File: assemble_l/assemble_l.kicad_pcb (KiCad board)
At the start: 2 copper layers, 134.9 x 119.3 mm, 61 parts, among them J1 Conn_01x02_Pin, SW1 SW_Push, SW10 SW_Push, SW11 SW_Push, SW12 SW_Push, SW13 SW_Push, SW14 SW_Push, SW15 SW_Push, SW16 SW_Push, SW17 SW_Push, SW18 SW_Push, SW19 SW_Push, SW2 SW_Push, SW20 SW_Push, SW21 SW_Push, SW22 SW_Push, SW23 SW_Push, SW24 SW_Push, SW25 SW_Push, SW26 SW_Push, SW27 SW_Push, SW28 SW_Push, SW3 SW_Push, SW4 SW_Push, SW5 SW_Push, SW6 SW_Push, SW7 SW_Push, SW8 SW_Push, SW9 SW_Push, U1 Micon_BLEMicroPro

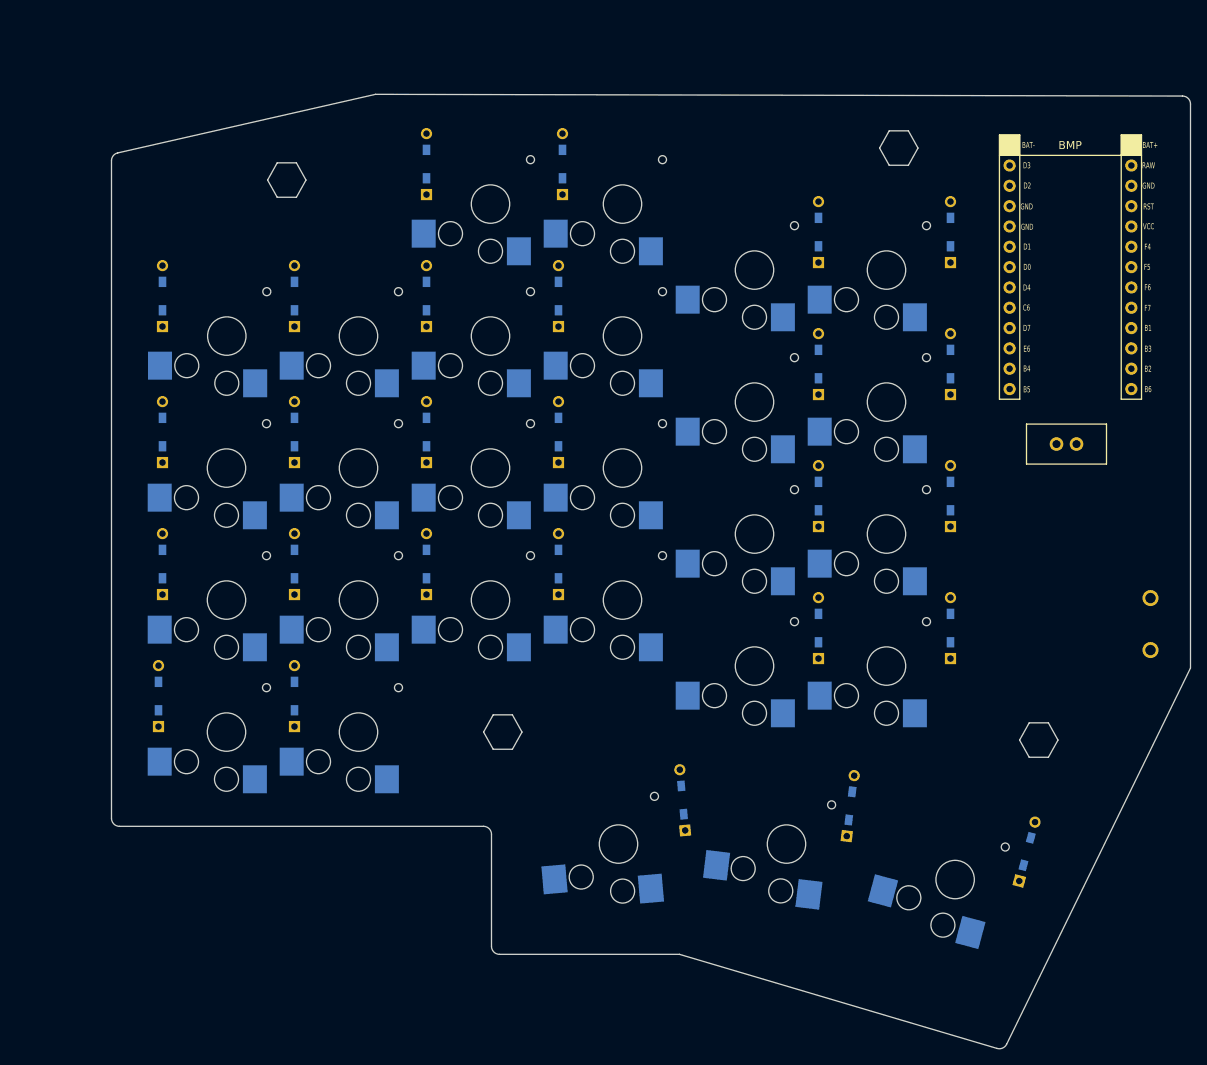
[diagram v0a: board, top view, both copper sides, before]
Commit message: feat: reallocate keys on left
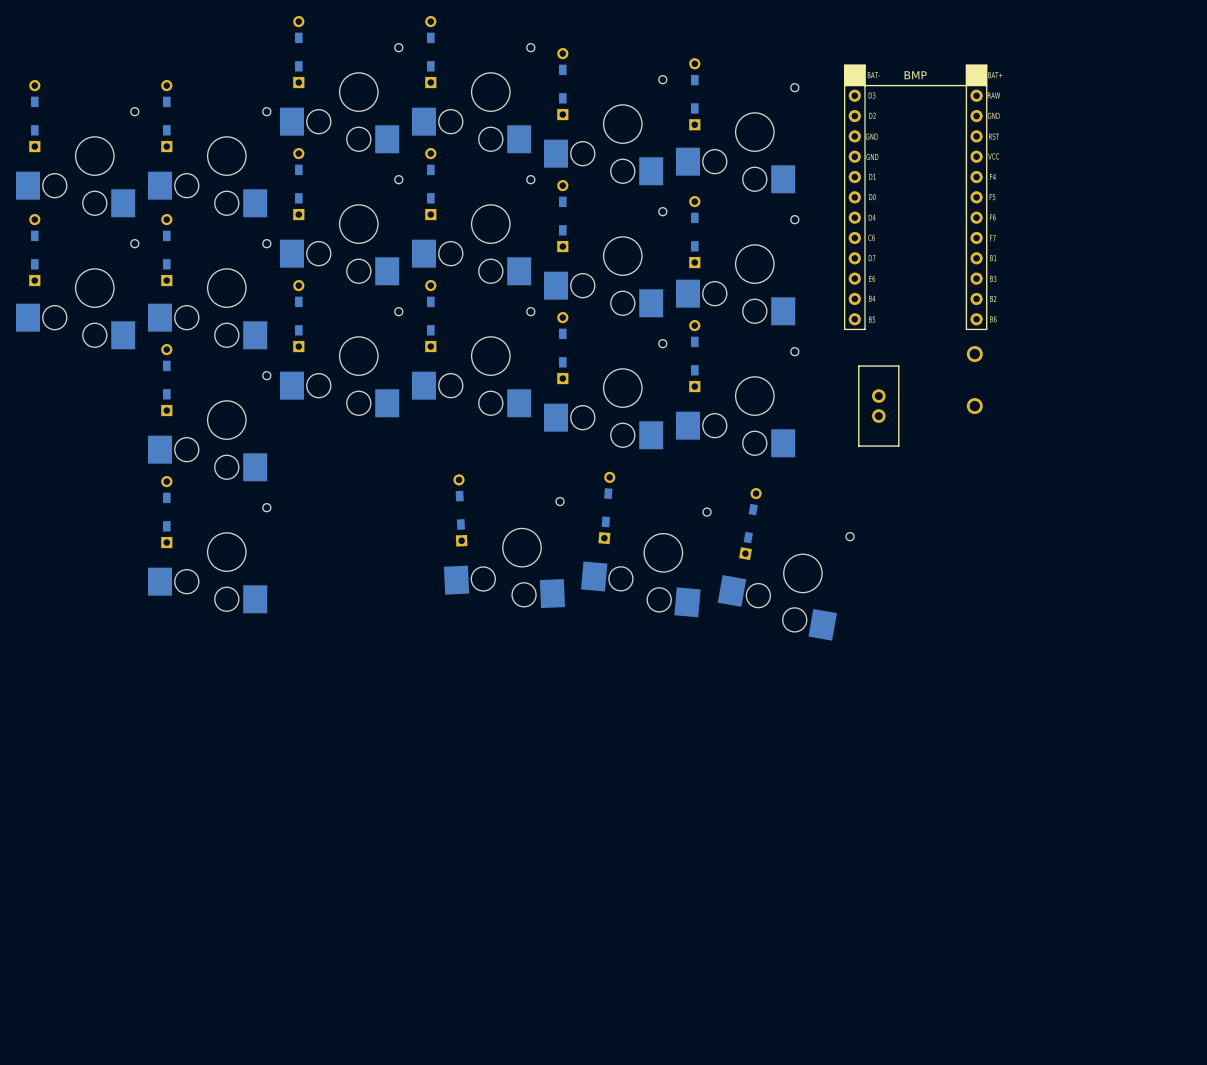
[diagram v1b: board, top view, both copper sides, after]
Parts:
- removed D22, D23, D24, D25, D26, D27: D, kbd_Parts:Diode_TH_SMD
- removed Ref** (x4): Val**, kbd_Hole:m2_Spacer_Hole_hex
- removed SW23, SW24, SW25, SW26, SW27: SW_Push, kbd_SW:Choc_v2_Hotswap_1u_16.5
- removed SW28: SW_Push, kbd_Parts:ResetSW
- SW22: footprint kbd_SW:Choc_v2_Hotswap_1u_16.5 -> kbd_Parts:ResetSW
- moved D6 99.7 mm to (77.0, 75.5)
- moved D19 88.6 mm to (143.0, 57.0)
- moved SW19 88.2 mm to (150.5, 61.0)
- moved SW6 84.6 mm to (84.5, 80.5)
- moved D5 81.5 mm to (77.0, 59.2)
- moved D14 68.7 mm to (126.5, 38.5)
- moved SW14 68.1 mm to (134.0, 43.5)
- moved SW5 66.0 mm to (84.5, 64.0)
- moved D20 65.7 mm to (143.0, 72.5)
- moved D12 65.2 mm to (110.0, 67.5)
- moved SW20 64.9 mm to (150.5, 77.5)
- moved D18 59.5 mm to (143.0, 39.8)
- moved SW3 54.6 mm to (84.5, 97.0)
- moved D3 54.3 mm to (77.0, 92.0)
- moved D11 53.4 mm to (110.0, 51.0)
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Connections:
- D10 pad 1: Row1 -> Row0
- D12 pad 1: Row1 -> Row2
- D13 pad 1: Row2 -> Row3
- D14 pad 1: Row2 -> Row0
- D15 pad 1: Row2 -> Row1
- D17 pad 1: Row2 -> Row3
- D18 pad 1: Row2 -> Row0
- D19 pad 1: Row3 -> Row1
- D2 pad 1: Row0 -> Row1
- D20 pad 1: Row3 -> Row2
- D3 pad 1: Row0 -> Row2
- D5 pad 1: Row0 -> Row1
- D6 pad 1: Row0 -> Row2
- D7 pad 1: Row1 -> Row0
- D9 pad 1: Row1 -> Row2
- SW11 pad 1: Col4 -> Col3
- SW12 pad 1: Col5 -> Col3
- SW13 pad 1: Col0 -> Col3
- SW14 pad 1: Col1 -> Col4
- SW15 pad 1: Col2 -> Col4
- SW16 pad 1: Col3 -> Col4
- SW19 pad 1: Col0 -> Col5
- SW2 pad 1: Col1 -> Col0
- SW20 pad 1: Col1 -> Col5
- SW21 pad 1: Col2 -> Col5
- SW22 pad 1: Col3 -> Reset
- SW22 pad 2: Net-(D22-A) -> GND
- SW3 pad 1: Col2 -> Col0
- SW4 pad 1: Col3 -> Col1
- SW5 pad 1: Col4 -> Col1
- SW6 pad 1: Col5 -> Col1
- SW7 pad 1: Col0 -> Col2
- SW8 pad 1: Col1 -> Col2
- U1 pad 11: Row4 -> unconnected-(U1-B4/PIN11-Pad11)
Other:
- board outline removed
